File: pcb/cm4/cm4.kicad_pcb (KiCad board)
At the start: 4 copper layers, 86.4 x 55.9 mm, 30 parts, among them J101 Conn_01x05, J102 Conn_01x08, J201 DF40C-100DS-0.4V_51_, J202 DF40C-100DS-0.4V_51_, J301 HR911130A, J401 Micro_SD_Card, U201 SN74LV1T34DBV, U301 TPD4EUSB30, U302 TPD4EUSB30, U401 RT9742GGJ5

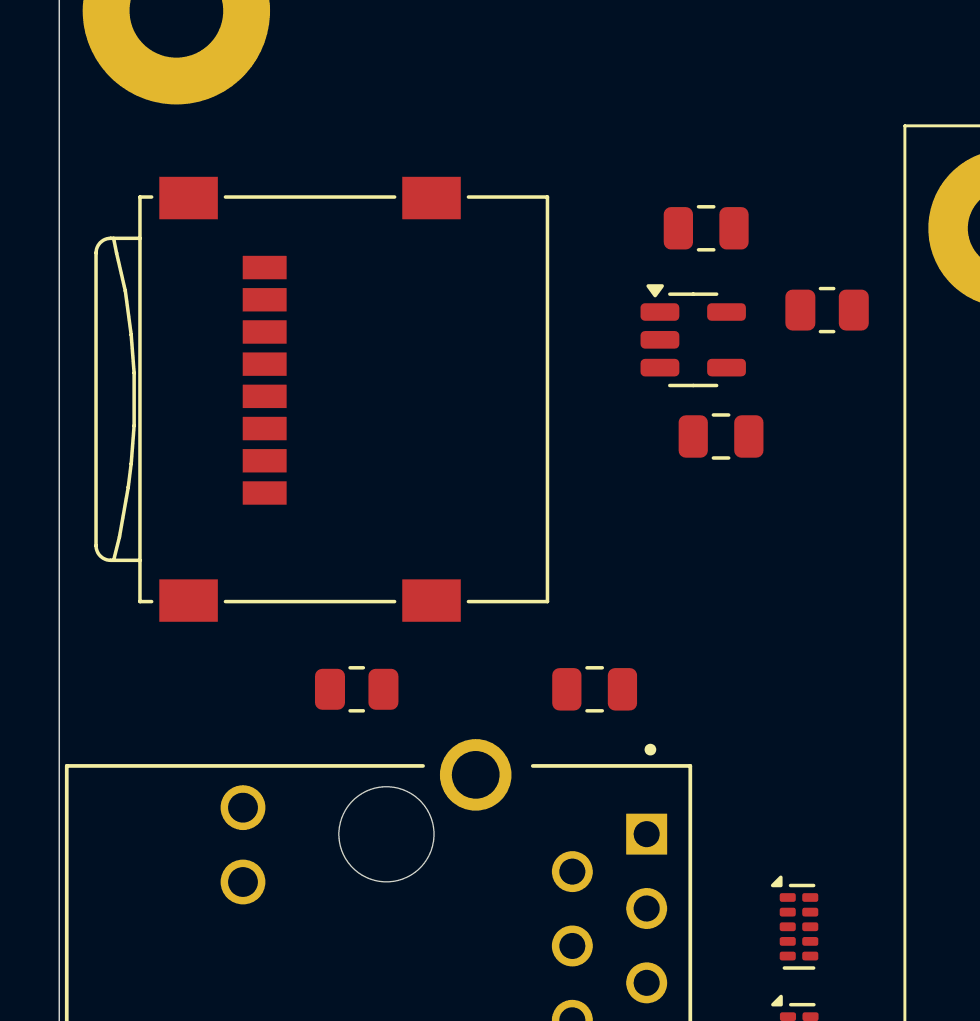
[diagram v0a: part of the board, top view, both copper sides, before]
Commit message: update cm4 board
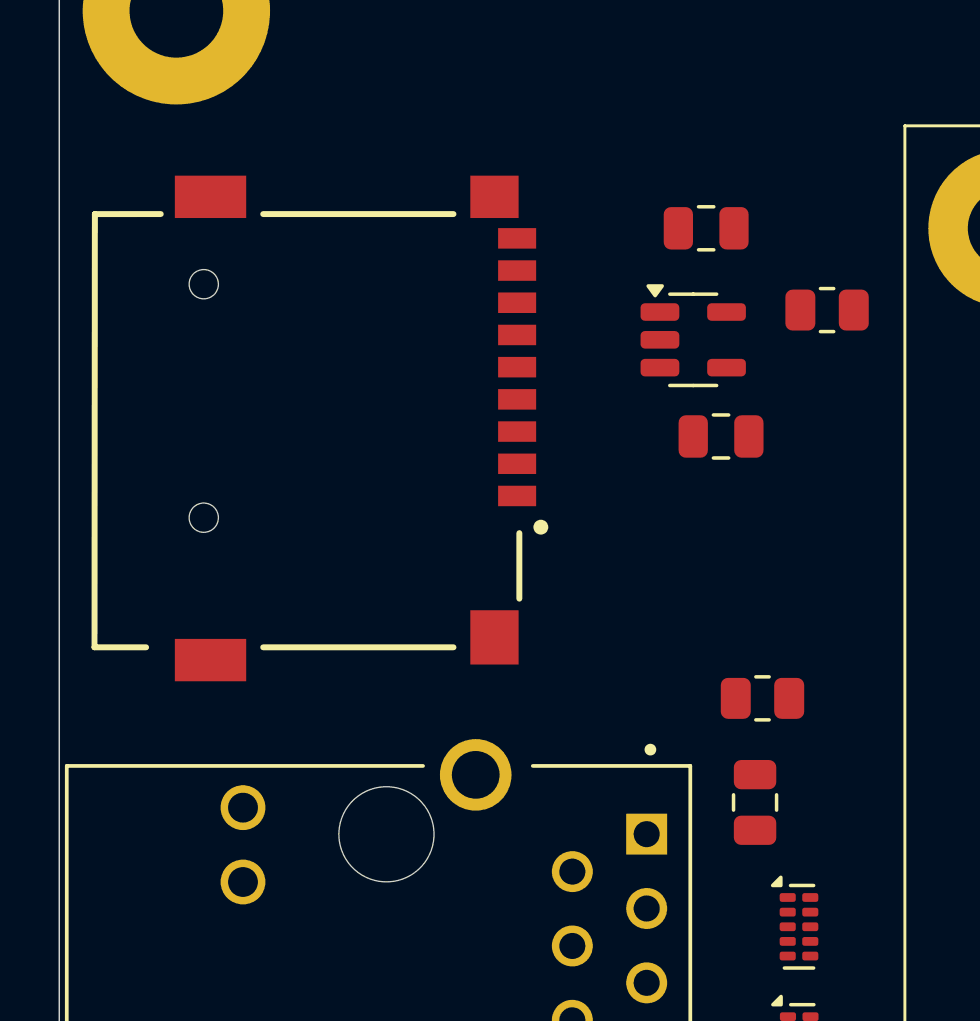
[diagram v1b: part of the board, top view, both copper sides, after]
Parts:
- removed J401: Micro_SD_Card, Connector_Card:microSD_HC_Wuerth_693072010801
- added MICRO_SD401: TF-01A, DF40C-100DS-0.4V_51_:TF-01A, F.Cu at (84.7, 94.5)
- moved R301 13.9 mm to (100.2, 103.7)
- moved C301 6.71 mm to (100.0, 107.2), turned to -90 degrees
